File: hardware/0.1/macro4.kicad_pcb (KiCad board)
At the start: 2 copper layers, 48 x 48 mm, 29 parts, among them J1 USB_C_Receptacle_USB2.0, Q1 BSS138, SW1 DFU, SW2 RST, SW3 CHERRY_MX, SW5 CHERRY_MX, SW6 CHERRY_MX, SW7 Rotary_Encoder_MX, U1 AP2112K-3.3, U2 STM32F072C8Tx

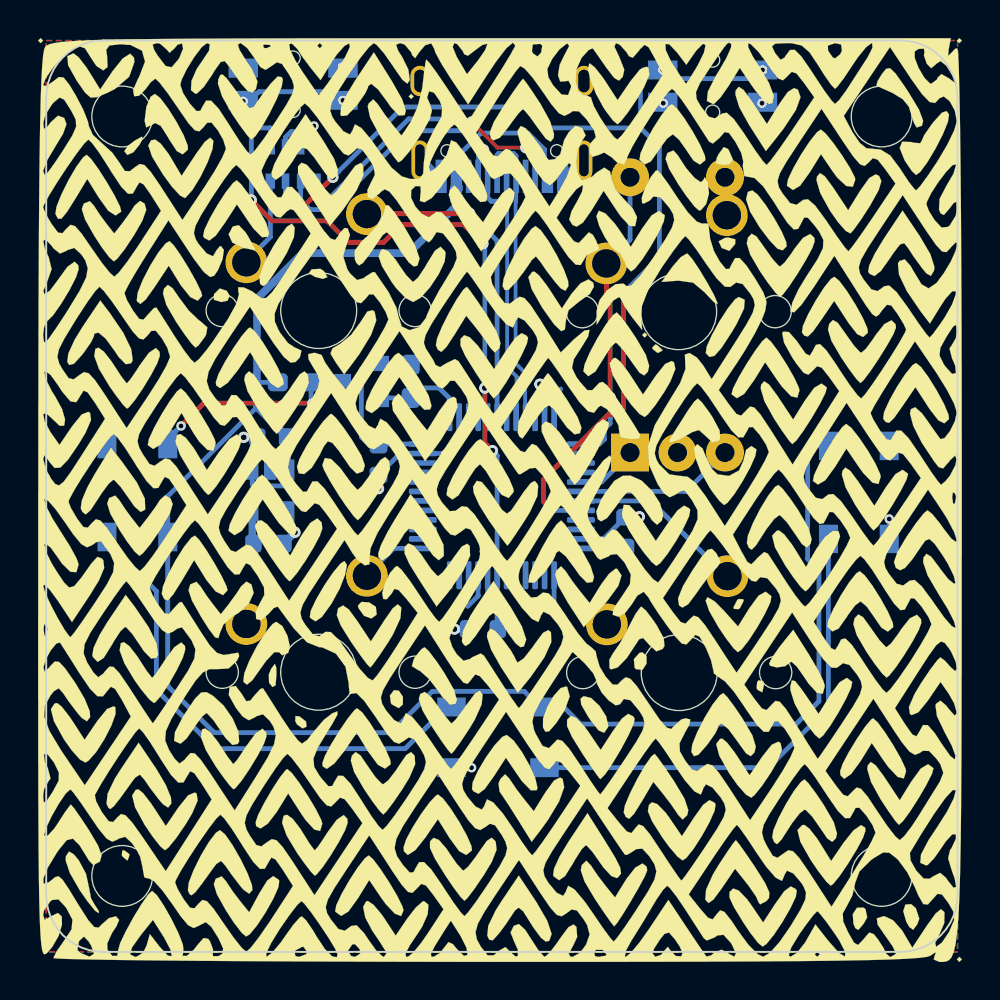
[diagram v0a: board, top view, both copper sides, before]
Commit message: v0.2
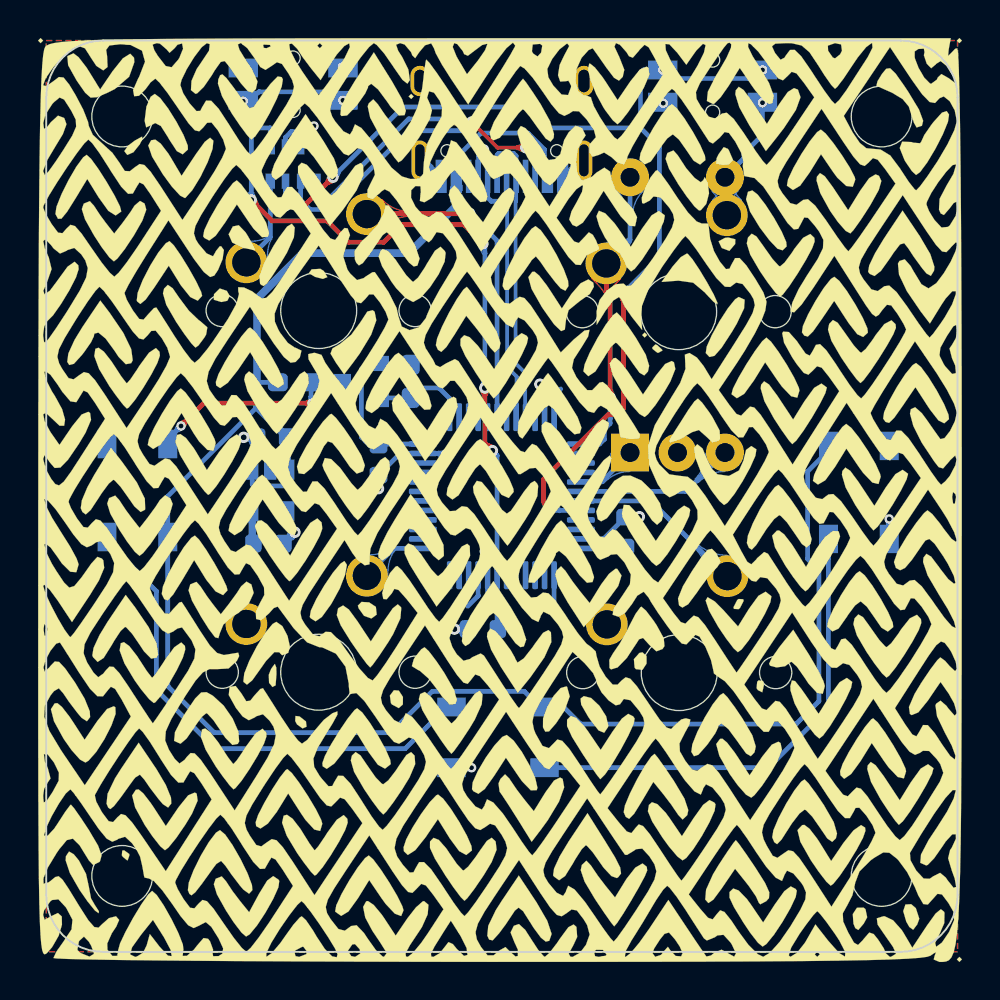
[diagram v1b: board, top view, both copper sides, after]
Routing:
- net +3V3: track 25.6 -> 30.4 mm
